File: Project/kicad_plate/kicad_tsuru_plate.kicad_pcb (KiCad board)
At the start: 2 copper layers, 209.6 x 57.1 mm, 0 parts

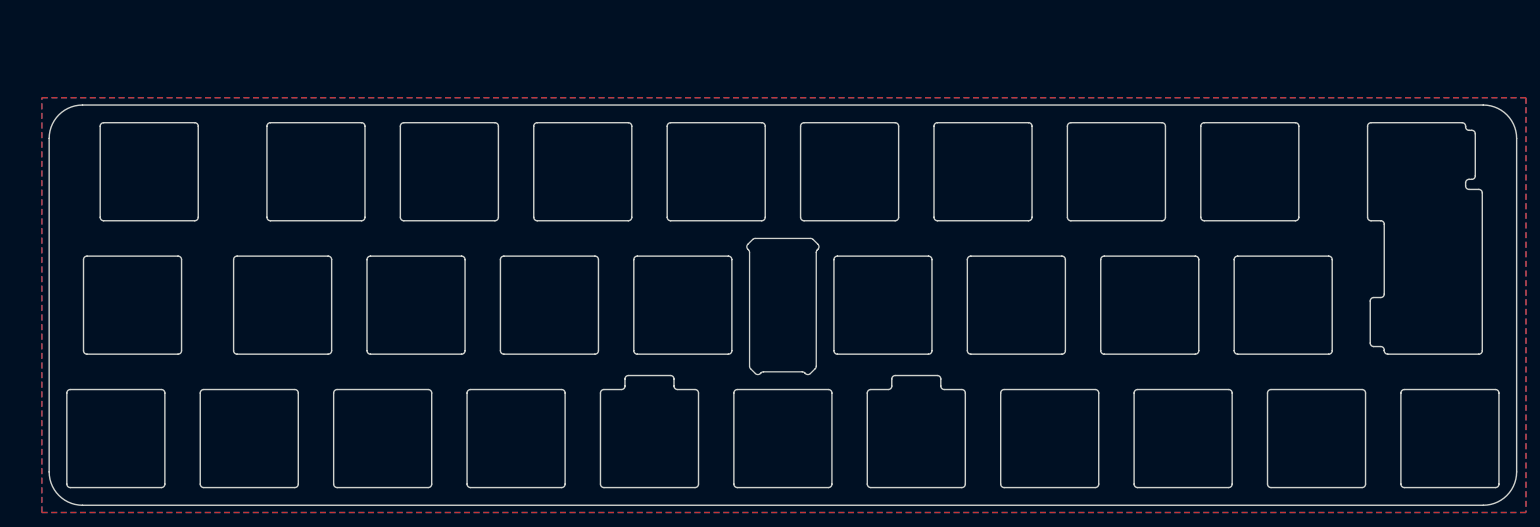
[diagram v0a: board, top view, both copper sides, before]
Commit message: fresh gerbers, various plate files
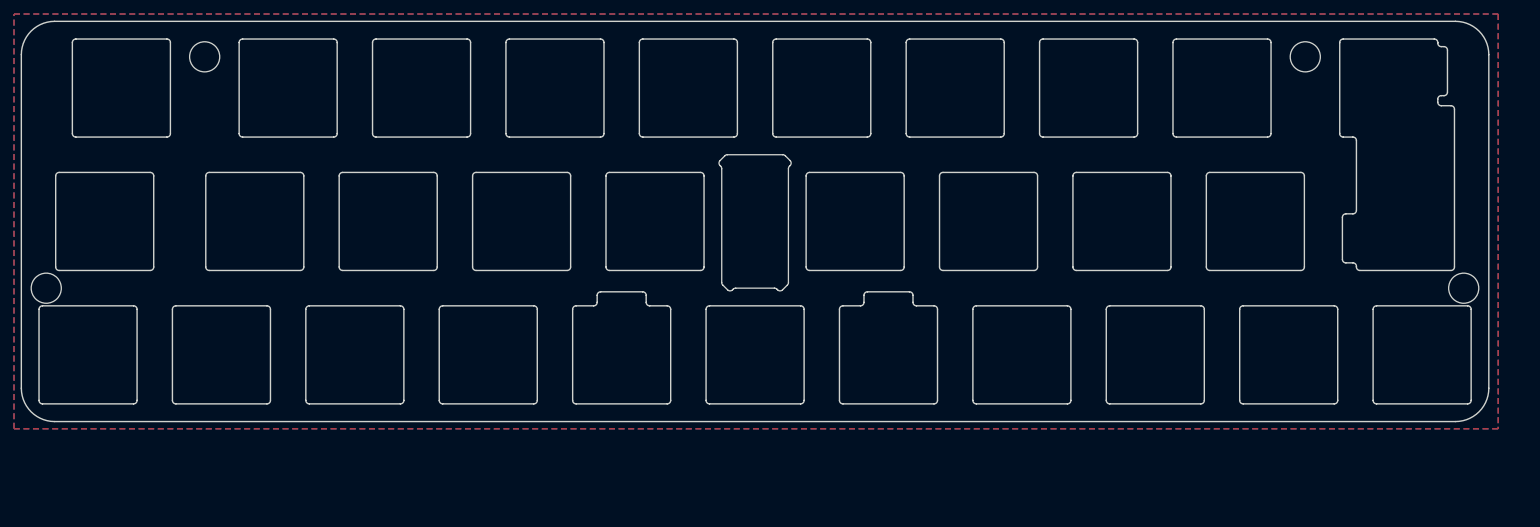
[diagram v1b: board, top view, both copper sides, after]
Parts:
- added REF**: MountingHole_4.3mm_M4, MountingHole:MountingHole_4.3mm_M4, F.Cu at (215.8, 58.6)
- added REF**: MountingHole_4.3mm_M4, MountingHole:MountingHole_4.3mm_M4, F.Cu at (36.1, 91.6)
- added REF**: MountingHole_4.3mm_M4, MountingHole:MountingHole_4.3mm_M4, F.Cu at (58.7, 58.6)
- added REF**: MountingHole_4.3mm_M4, MountingHole:MountingHole_4.3mm_M4, F.Cu at (238.5, 91.6)
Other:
- board size 209.6 x 57.1 mm -> 209.6 x 57.2 mm
